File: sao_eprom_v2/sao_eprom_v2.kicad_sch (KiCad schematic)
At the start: 8 parts, among them J1 USB_C_Receptacle_USB2.0, J2 Conn_01x03, U1 RP2040, X1 YSO110TR

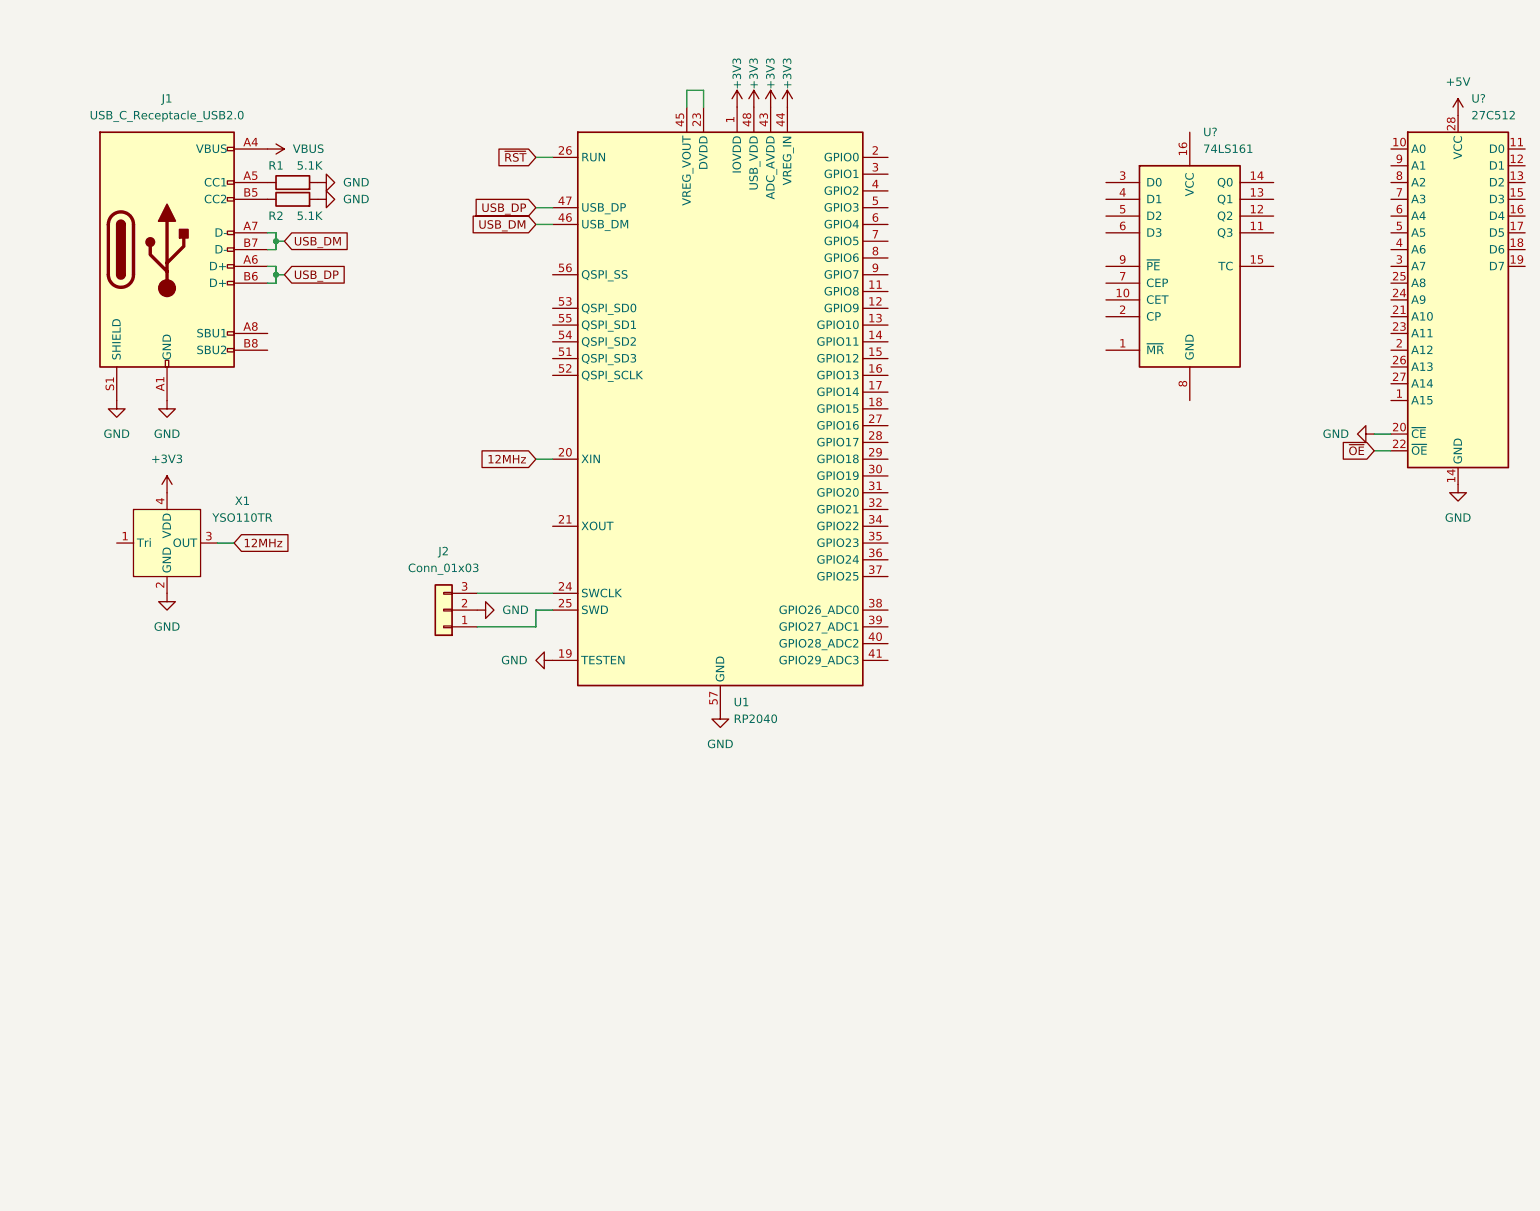
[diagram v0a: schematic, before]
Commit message: More works on eprom v2
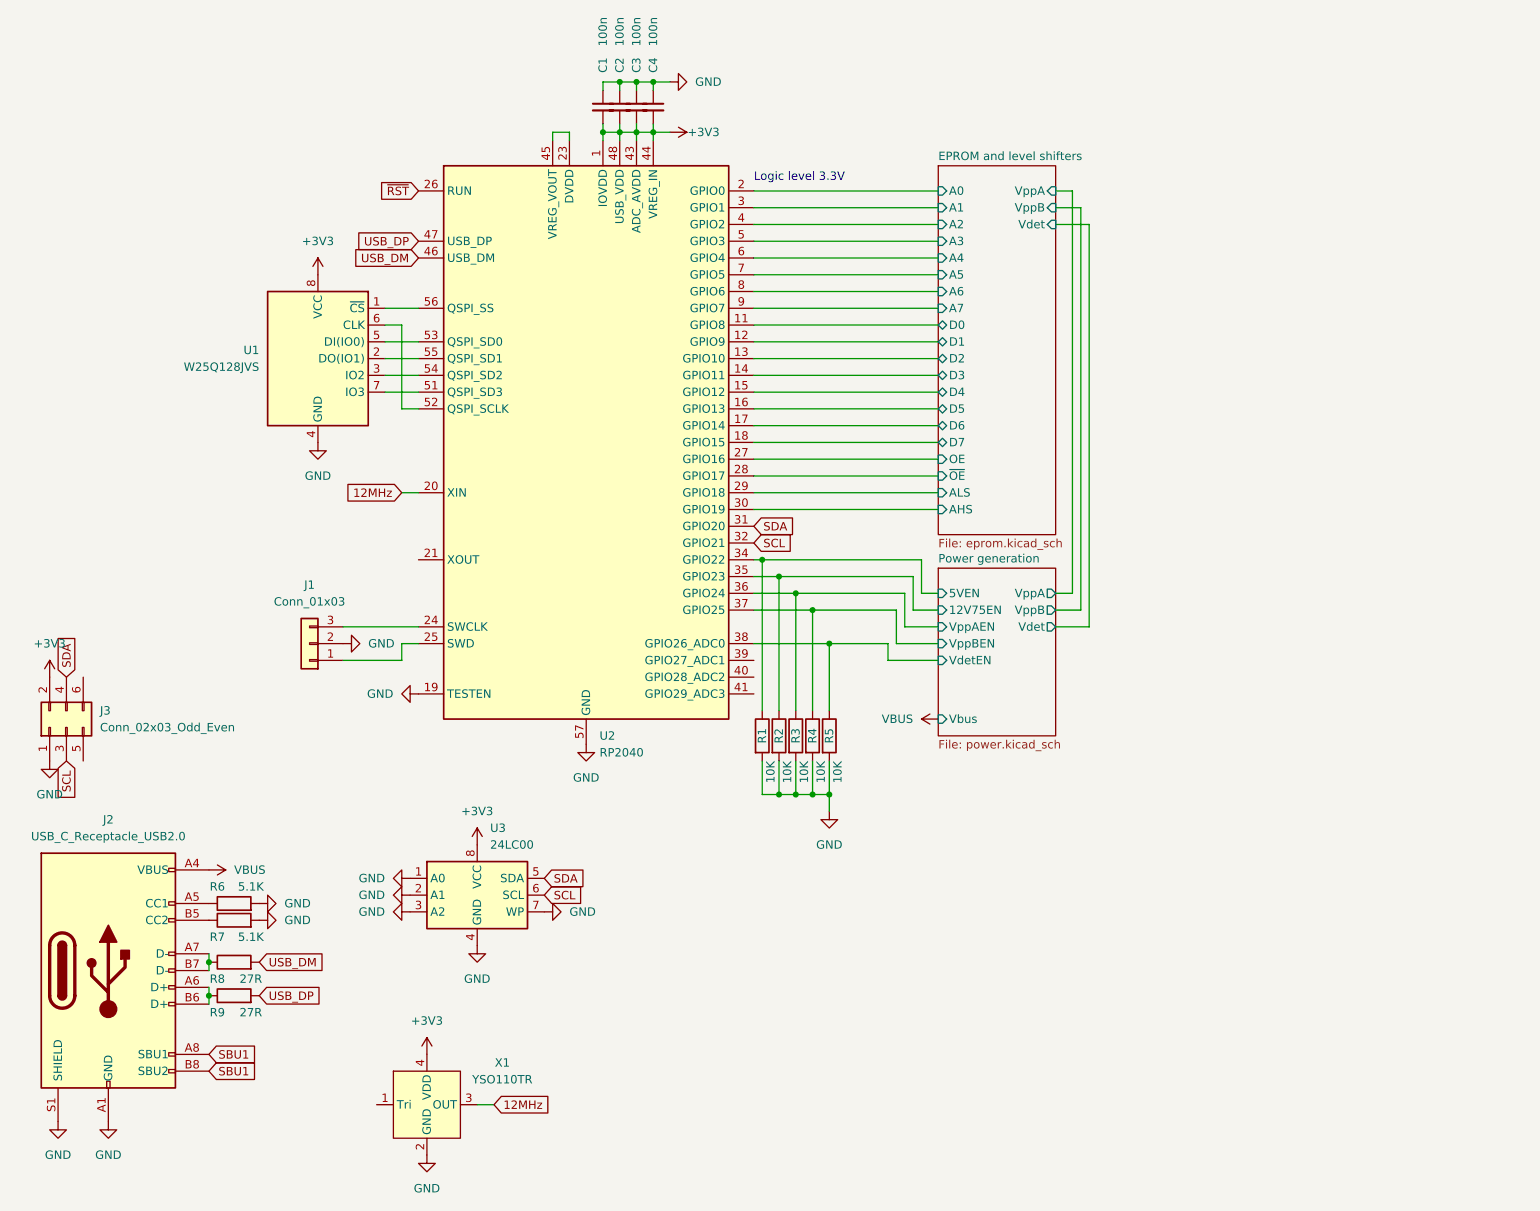
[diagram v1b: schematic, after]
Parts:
- removed U?: 74LS161, symbol 74xx:74LS161
- removed U?: 27C512, Package_DIP:DIP-28_W15.24mm, symbol Memory_EPROM:27C512
- added C1, C2, C3, C4: 100n, Capacitor_SMD:C_0402_1005Metric, symbol Device:C_Small
- added J3: Conn_02x03_Odd_Even, Connector_PinHeader_2.54mm:PinHeader_2x03_P2.54mm_Vertical, symbol Connector_Generic:Conn_02x03_Odd_Even
- added R1, R2, R3, R4, R5: 10K, Resistor_SMD:R_0402_1005Metric_Pad0.72x0.64mm_HandSolder, symbol Device:R
- added R8, R9: 27R, Resistor_SMD:R_0402_1005Metric_Pad0.72x0.64mm_HandSolder, symbol Device:R
- added U1: W25Q128JVS, Package_SO:SOIC-8_5.23x5.23mm_P1.27mm, symbol Memory_Flash:W25Q128JVS
- added U3: 24LC00, Package_SO:SOIC-8_3.9x4.9mm_P1.27mm, symbol Memory_EEPROM:24LC00
- J2: renamed from J1; footprint (none) -> Connector_USB:USB_C_Receptacle_G-Switch_GT-USB-7010ASV
- R6: renamed from R1; footprint Resistor_THT:R_Axial_DIN0207_L6.3mm_D2.5mm_P10.16mm_Horizontal -> Resistor_SMD:R_0402_1005Metric_Pad0.72x0.64mm_HandSolder
- R7: renamed from R2; footprint Resistor_THT:R_Axial_DIN0207_L6.3mm_D2.5mm_P10.16mm_Horizontal -> Resistor_SMD:R_0402_1005Metric_Pad0.72x0.64mm_HandSolder
- renumbered J2 to J1, U1 to U2
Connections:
- net +3V3: now also C1.2, C2.2, C3.2, C4.2, J3.2 (Pin_2), U1.8 (VCC), U3.8 (VCC)
- net GND: now also C1.1, C2.1, C3.1, C4.1, J3.1 (Pin_1), R1.2, R2.2, R3.2, R4.2, R5.2, U1.4 (GND), U3.1 (A0), U3.2 (A1), U3.3 (A2), U3.4 (GND), U3.7 (WP)
- net USB_DM: now also R8.2; no longer J2.A7 (D-), J2.B7 (D-)
- net USB_DP: now also R9.2; no longer J2.A6 (D+), J2.B6 (D+)
- net SBU1: now reaches J2.A8 (SBU1)
- net SBU1: now also J2.B8 (SBU2)
- net EPROM and level shifters/D0: now reaches U2.11 (GPIO8)
- net EPROM and level shifters/D1: now reaches U2.12 (GPIO9)
- net EPROM and level shifters/D2: now reaches U2.13 (GPIO10)
- net EPROM and level shifters/D3: now reaches U2.14 (GPIO11)
- net EPROM and level shifters/D4: now reaches U2.15 (GPIO12)
- net EPROM and level shifters/D5: now reaches U2.16 (GPIO13)
- net EPROM and level shifters/D6: now reaches U2.17 (GPIO14)
- net EPROM and level shifters/D7: now reaches U2.18 (GPIO15)
- net EPROM and level shifters/A0: now reaches U2.2 (GPIO0)
- net EPROM and level shifters/OE: now reaches U2.27 (GPIO16)
- net EPROM and level shifters/~{OE}: now reaches U2.28 (GPIO17)
- net EPROM and level shifters/ALS: now reaches U2.29 (GPIO18)
- net EPROM and level shifters/A1: now reaches U2.3 (GPIO1)
- net EPROM and level shifters/AHS: now reaches U2.30 (GPIO19)
- net SDA: now reaches U2.31 (GPIO20)
- net SDA: now also J3.4 (Pin_4), U3.5 (SDA)
- net SCL: now reaches U2.32 (GPIO21)
- net SCL: now also J3.3 (Pin_3), U3.6 (SCL)
- net Power generation/5VEN: now reaches U2.34 (GPIO22)
- net Power generation/5VEN: now also R1.1
- net Power generation/12V75EN: now reaches U2.35 (GPIO23)
- net Power generation/12V75EN: now also R2.1
- net Power generation/VppAEN: now reaches U2.36 (GPIO24)
- net Power generation/VppAEN: now also R3.1
- net Power generation/VppBEN: now reaches U2.37 (GPIO25)
- net Power generation/VppBEN: now also R4.1
- net Power generation/VdetEN: now reaches U2.38 (GPIO26_ADC0)
- net Power generation/VdetEN: now also R5.1
- net EPROM and level shifters/A2: now reaches U2.4 (GPIO2)
- net EPROM and level shifters/A3: now reaches U2.5 (GPIO3)
- net at U2.51 (QSPI_SD3): now also U1.7 (IO3)
- net at U2.52 (QSPI_SCLK): now also U1.6 (CLK)
- net at U2.53 (QSPI_SD0): now also U1.5 (DI(IO0))
- net at U2.54 (QSPI_SD2): now also U1.3 (IO2)
- net at U2.55 (QSPI_SD1): now also U1.2 (DO(IO1))
- net at U2.56 (QSPI_SS): now also U1.1 (~{CS})
- net EPROM and level shifters/A4: now reaches U2.6 (GPIO4)
- net EPROM and level shifters/A5: now reaches U2.7 (GPIO5)
- net EPROM and level shifters/A6: now reaches U2.8 (GPIO6)
- net EPROM and level shifters/A7: now reaches U2.9 (GPIO7)
- new net: J2.A6 (D+), J2.B6 (D+), R9.1
- new net: J2.A7 (D-), J2.B7 (D-), R8.1
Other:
- added sheet EPROM and level shifters (eprom.kicad_sch)
- added sheet Power generation (power.kicad_sch)
- note added: "Logic level 3.3V"
- moved on the sheet: J1, J2, R6, R7, U2, X1
